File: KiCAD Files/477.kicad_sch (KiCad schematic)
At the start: 28 parts, among them IC1 W25N01GVSFIG, IC2 W25N01GVSFIG, IC3 W25N01GVSFIG, IC4 W25N01GVSFIG, IC6 USBLC6-2SC6, J1 BM06B-SRSS-TBT_LF__SN_, J2 6364372-2, J5 BM07B-SRSS-TB_LF__SN_, J6 BM09B-SRSS-TB_LF__SN_

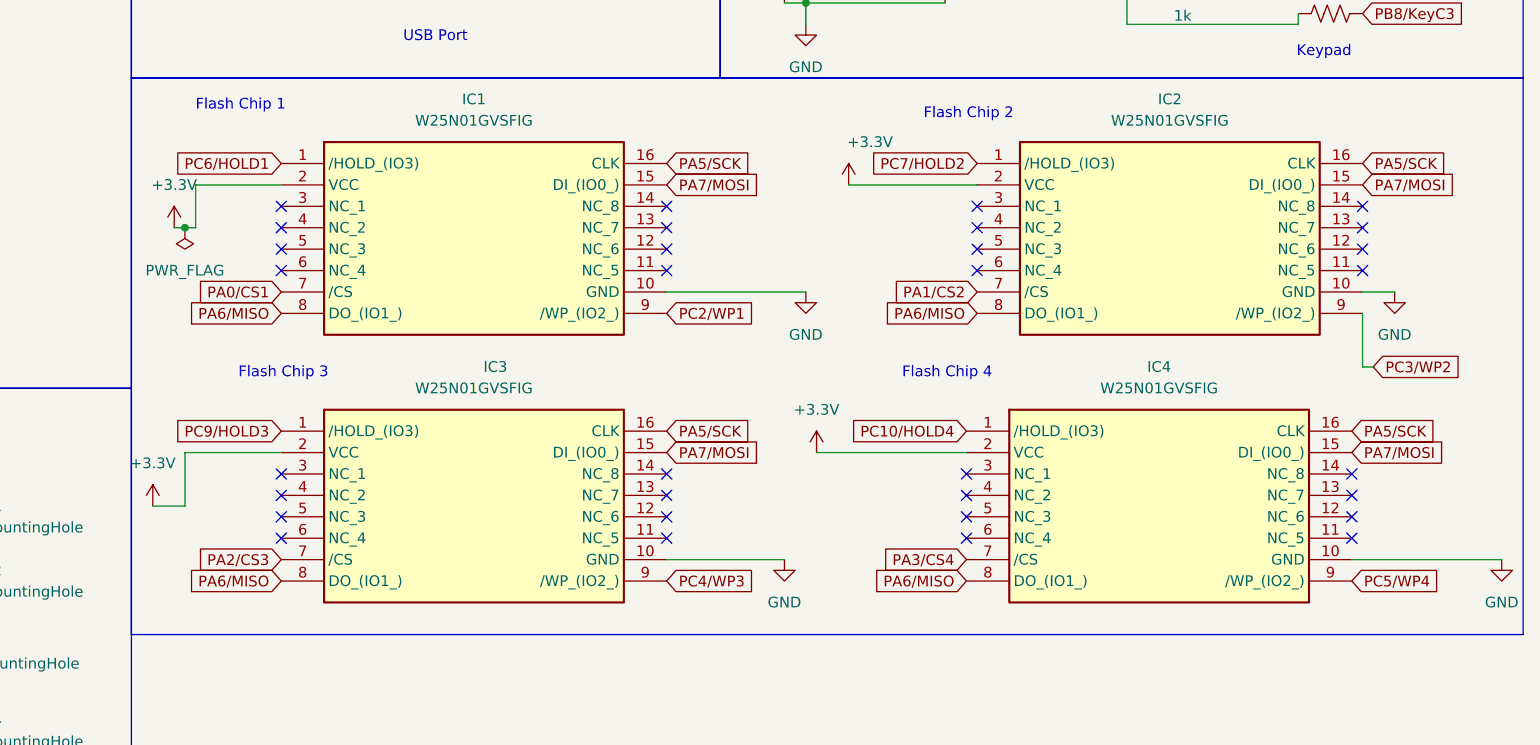
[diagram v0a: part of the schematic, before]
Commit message: finished file
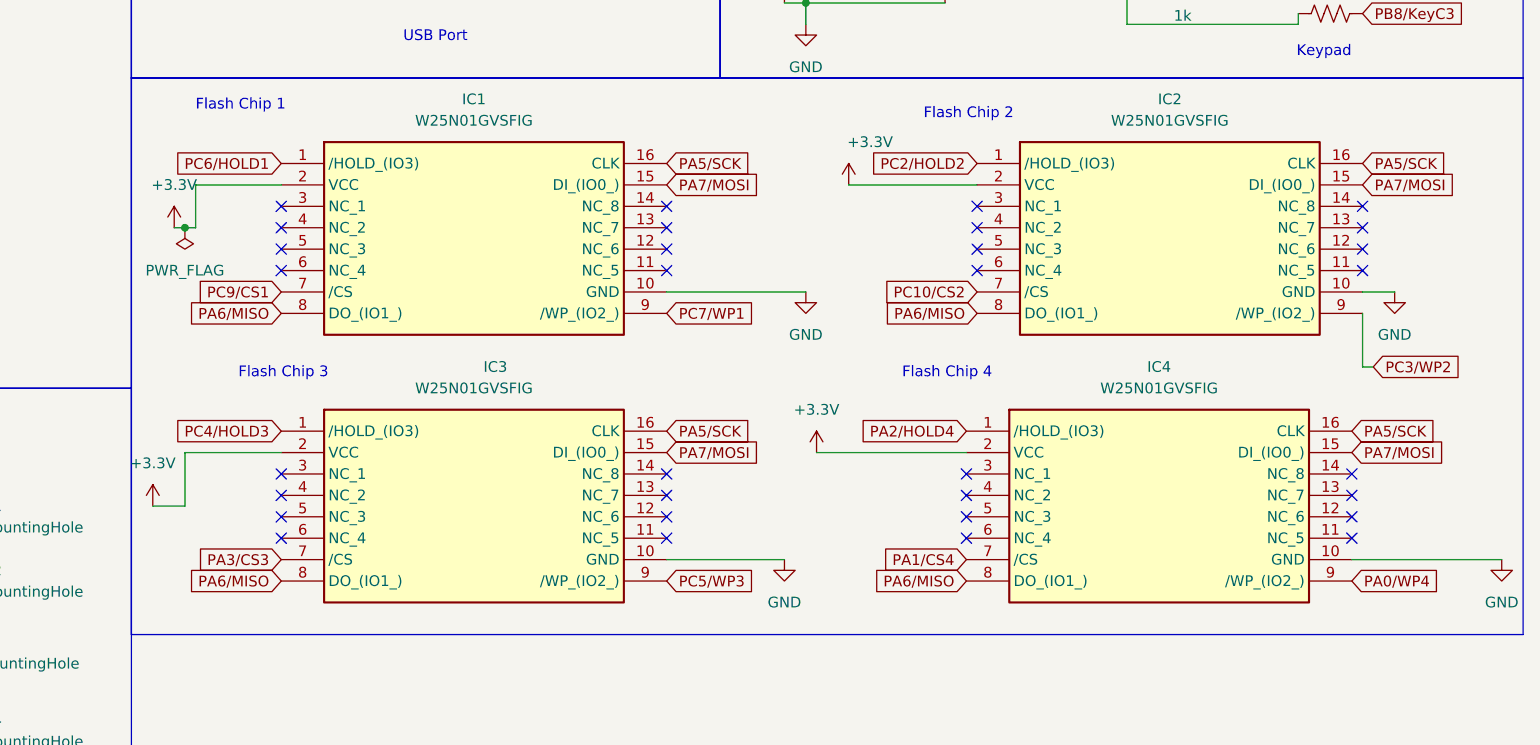
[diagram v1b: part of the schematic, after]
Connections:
- net PA0/CS1 renamed PC9/CS1
- net PA1/CS2 renamed PC10/CS2
- net PA2/CS3 renamed PA3/CS3
- net PA3/CS4 renamed PA1/CS4
- net PC10/HOLD4 renamed PA2/HOLD4
- net PC2/WP1 renamed PC7/WP1
- net PC4/WP3 renamed PC5/WP3
- net PC5/WP4 renamed PA0/WP4
- net PC7/HOLD2 renamed PC2/HOLD2
- net PC9/HOLD3 renamed PC4/HOLD3
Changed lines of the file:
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@@
 		)
 	)
-	(global_label "PC5{slash}WP4"
+	(global_label "PA0{slash}WP4"
 		(shape input)
 		(at 264.16 158.75 0)
@@
 		)
 		(property "Intersheetrefs" "${INTERSHEET_REFS}"
-			(at 276.1561 158.75 0)
-			(effects
-				(font
-					(size 1.27 1.27)
-				)
-				(justify left)
-				(hide yes)
-			)
-		)
-	)
-	(global_label "PA0{slash}CS1"
+			(at 275.9747 158.75 0)
+			(effects
+				(font
+					(size 1.27 1.27)
+				)
+				(justify left)
+				(hide yes)
+			)
+		)
+	)
+	(global_label "PC9{slash}CS1"
 		(shape input)
 		(at 137.16 124.46 180)
@@
 		)
 		(property "Intersheetrefs" "${INTERSHEET_REFS}"
-			(at 125.5872 124.46 0)
+			(at 125.4058 124.46 0)
 			(effects
 				(font
@@
 		)
 	)
-	(global_label "PC10{slash}HOLD4"
+	(global_label "PA2{slash}HOLD4"
 		(shape input)
 		(at 218.44 140.97 180)
@@
 		)
 		(property "Intersheetrefs" "${INTERSHEET_REFS}"
-			(at 202.9967 140.97 0)
+			(at 204.3876 140.97 0)
 			(effects
 				(font
@@
 		)
 	)
-	(global_label "PC7{slash}HOLD2"
+	(global_label "PC2{slash}HOLD2"
 		(shape input)
 		(at 219.71 109.22 180)
@@
 		)
 	)
-	(global_label "PA2{slash}CS3"
+	(global_label "PA3{slash}CS3"
 		(shape input)
 		(at 137.16 156.21 180)
@@
 		)
 	)
-	(global_label "PA1{slash}CS2"
+	(global_label "PC10{slash}CS2"
 		(shape input)
 		(at 219.71 124.46 180)
@@
 		)
 		(property "Intersheetrefs" "${INTERSHEET_REFS}"
-			(at 208.1372 124.46 0)
-			(effects
-				(font
-					(size 1.27 1.27)
-				)
-				(justify right)
-				(hide yes)
-			)
-		)
-	)
-	(global_label "PC2{slash}WP1"
+			(at 206.7463 124.46 0)
+			(effects
+				(font
+					(size 1.27 1.27)
+				)
+				(justify right)
+				(hide yes)
+			)
+		)
+	)
+	(global_label "PC7{slash}WP1"
 		(shape input)
 		(at 182.88 127 0)
@@
 		)
 	)
-	(global_label "PC9{slash}HOLD3"
+	(global_label "PC4{slash}HOLD3"
 		(shape input)
 		(at 137.16 140.97 180)
@@
 		)
 	)
-	(global_label "PA3{slash}CS4"
+	(global_label "PA1{slash}CS4"
 		(shape input)
 		(at 218.44 156.21 180)
@@
 		)
 	)
-	(global_label "PC4{slash}WP3"
+	(global_label "PC5{slash}WP3"
 		(shape input)
 		(at 182.88 158.75 0)
